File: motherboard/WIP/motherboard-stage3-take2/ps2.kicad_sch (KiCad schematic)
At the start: 24 parts, among them U1 74HCT32, U2 74HCT14, U3 74HCT595, U4 74HCT595, U5 74HCT14, U6 74HCT573, U7 74HCT595, U8 74HCT595, U9 74HCT573

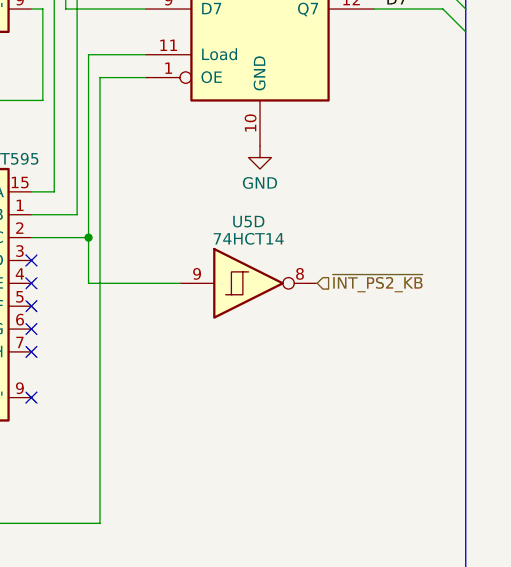
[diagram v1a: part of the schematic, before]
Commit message: Ordered stage 2!
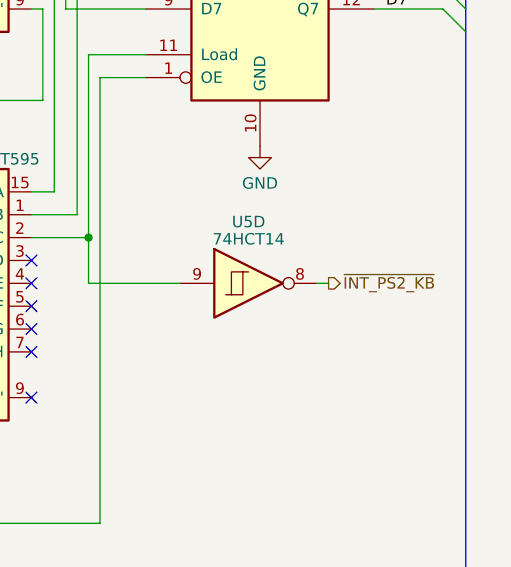
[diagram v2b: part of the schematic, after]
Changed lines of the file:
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@@
+	(wire
+		(pts
+			(xy 254 77.47) (xy 255.27 77.47)
+		)
+		(stroke
+			(width 0)
+			(type default)
+		)
+	)
 	(wire
 		(pts
@@
 	)
 	(hierarchical_label "~{INT_PS2_KB}"
-		(shape input)
-		(at 254 77.47 0)
-		(fields_autoplaced yes)
-		(effects
+		(shape output)
+		(at 255.27 77.47 0)
+		(fields_autoplaced yes)
+		(effects
